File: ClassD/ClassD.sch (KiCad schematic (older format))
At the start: 35 parts, among them P1 CONN_01X02, P2 BNC, P3 BNC, SW1 SPST, U1 AP1117E50G-13, U2 TPA2008D2

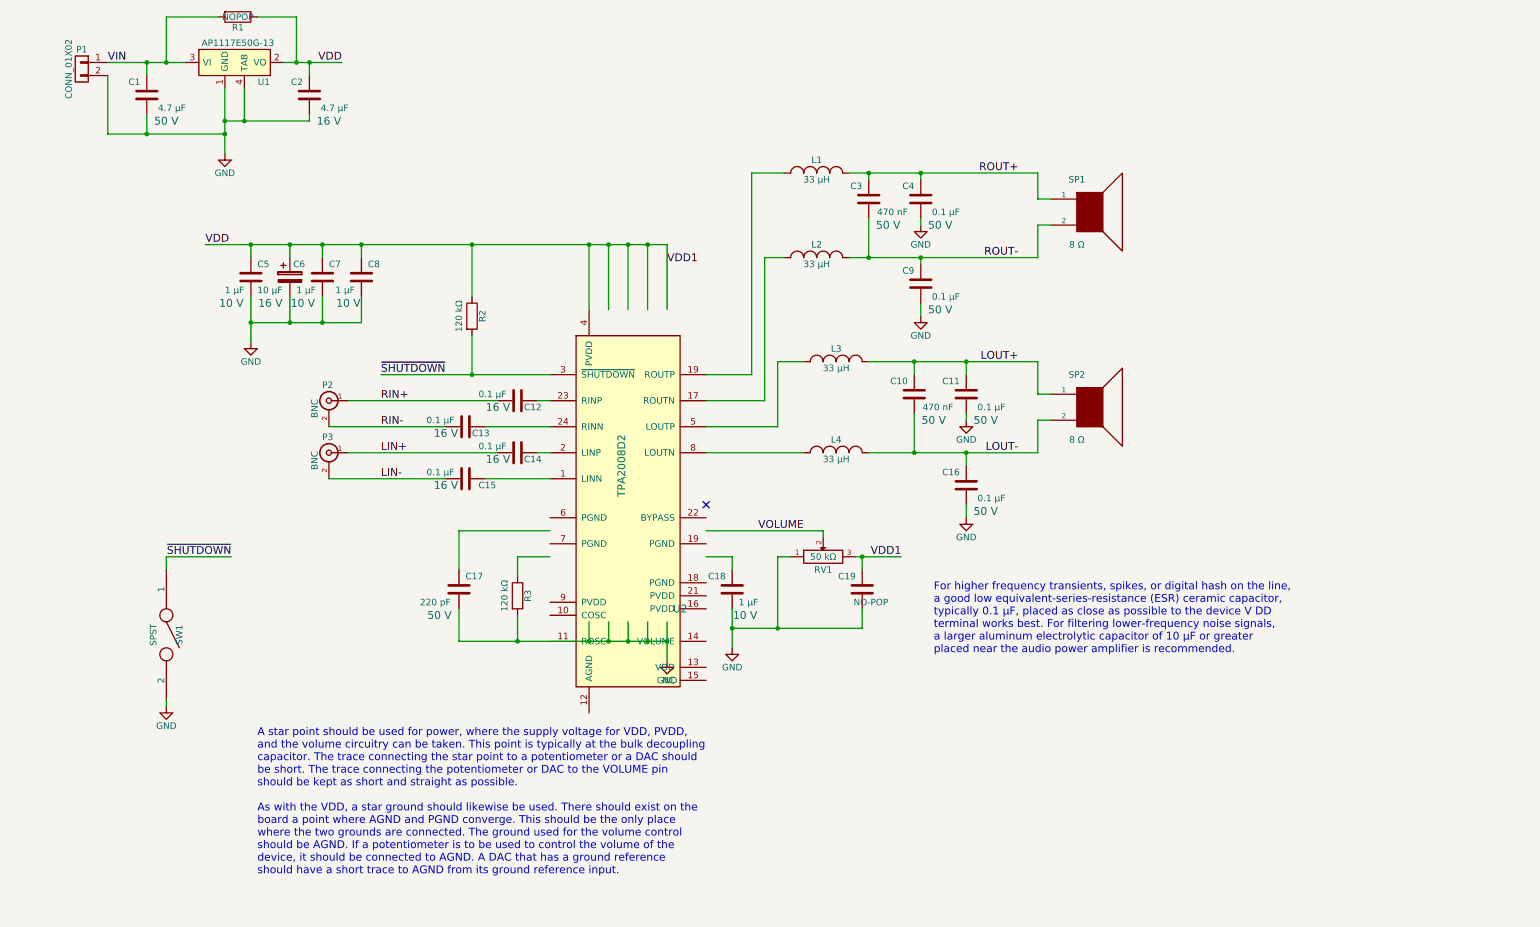
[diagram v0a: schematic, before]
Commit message: Started the layout
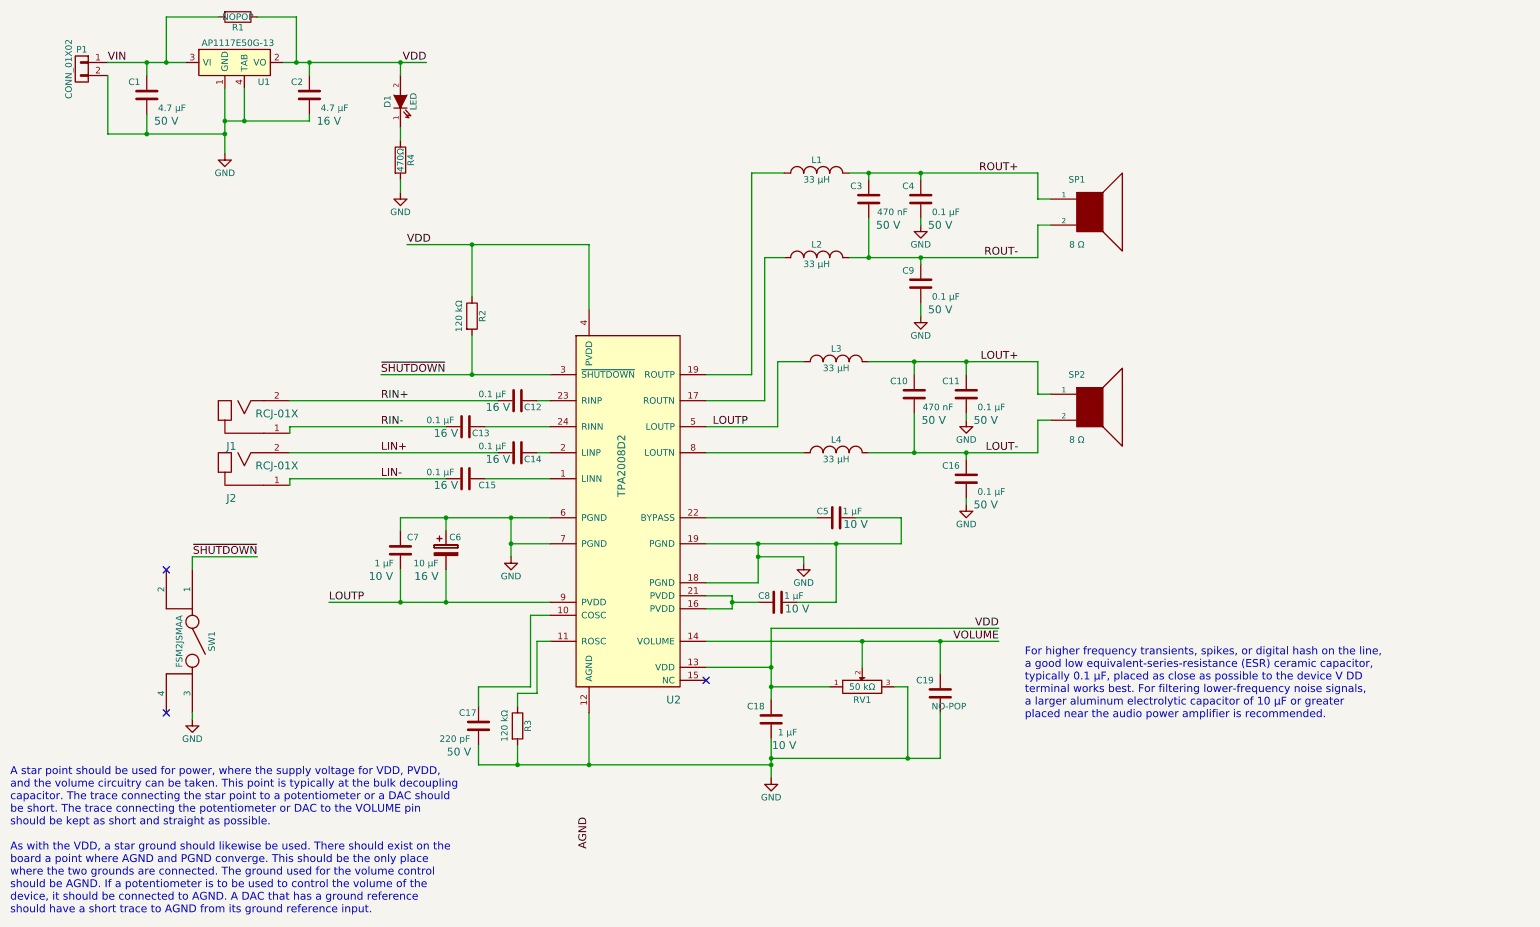
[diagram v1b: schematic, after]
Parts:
- removed P2, P3: BNC, symbol BNC
- removed SW1: SPST, symbol SPST
- added D1: LED, LEDs:LED_0805, symbol LED
- added J1, J2: RCJ-01X, LoudMouth-ClassD:RCJ-01X, symbol RCJ-01X
- added R4: 470Ω, Resistors_SMD:R_0805, symbol R
- added SW1: FSM2JSMAA, LoudMouth-ClassD:FSM2JSMAA, symbol FSM2JSMAA
- C19: ConradPN (none) -> Value; Link (none) -> Value; On-Hand (none) -> Yes; Voltage (none) -> Value
- C6: footprint (none) -> Capacitors_SMD:c_elec_4x5.3
- L1, L2, L3, L4: footprint (none) -> LoudMouth-ClassD:SRN3051
- P1: footprint (none) -> Pin_Headers:Pin_Header_Straight_1x02
- R1: footprint (none) -> Resistors_SMD:R_0805; ConradPN (none) -> Value; DigiKeyPN (none) -> Value; Link (none) -> Value; On-Hand (none) -> No; Voltage (none) -> Value
- R2, R3: footprint (none) -> Resistors_SMD:R_0805
- RV1: footprint (none) -> LoudMouth-ClassD:EVUE-POT; Fieldname Value -> (none); Link (none) -> Value; On-Hand (none) -> No
- SP1, SP2: footprint (none) -> Pin_Headers:Pin_Header_Straight_1x02; On-Hand (none) -> Yes
- U1: footprint (none) -> TO_SOT_Packages_SMD:SOT-223
- U2: footprint (none) -> LoudMouth-ClassD:24-TSSOP-PowerPad; ConradPN Value -> 1071052 - 62; Link (none) -> https://www.conrad.de/de/linear-ic-verstaerker-audio-texas-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; On-Hand (none) -> No
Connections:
- net labels added: AGND, LOUTP
- net labels removed: VDD1
- wire segments 101 -> 116
- no-connect marks 1 -> 3
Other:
- moved on the sheet: C16, C17, C18, C19, C5, C6, C7, C8, R3, RV1
